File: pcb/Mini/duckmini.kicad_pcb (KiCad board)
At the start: 2 copper layers, 126.9 x 99.3 mm, 42 parts

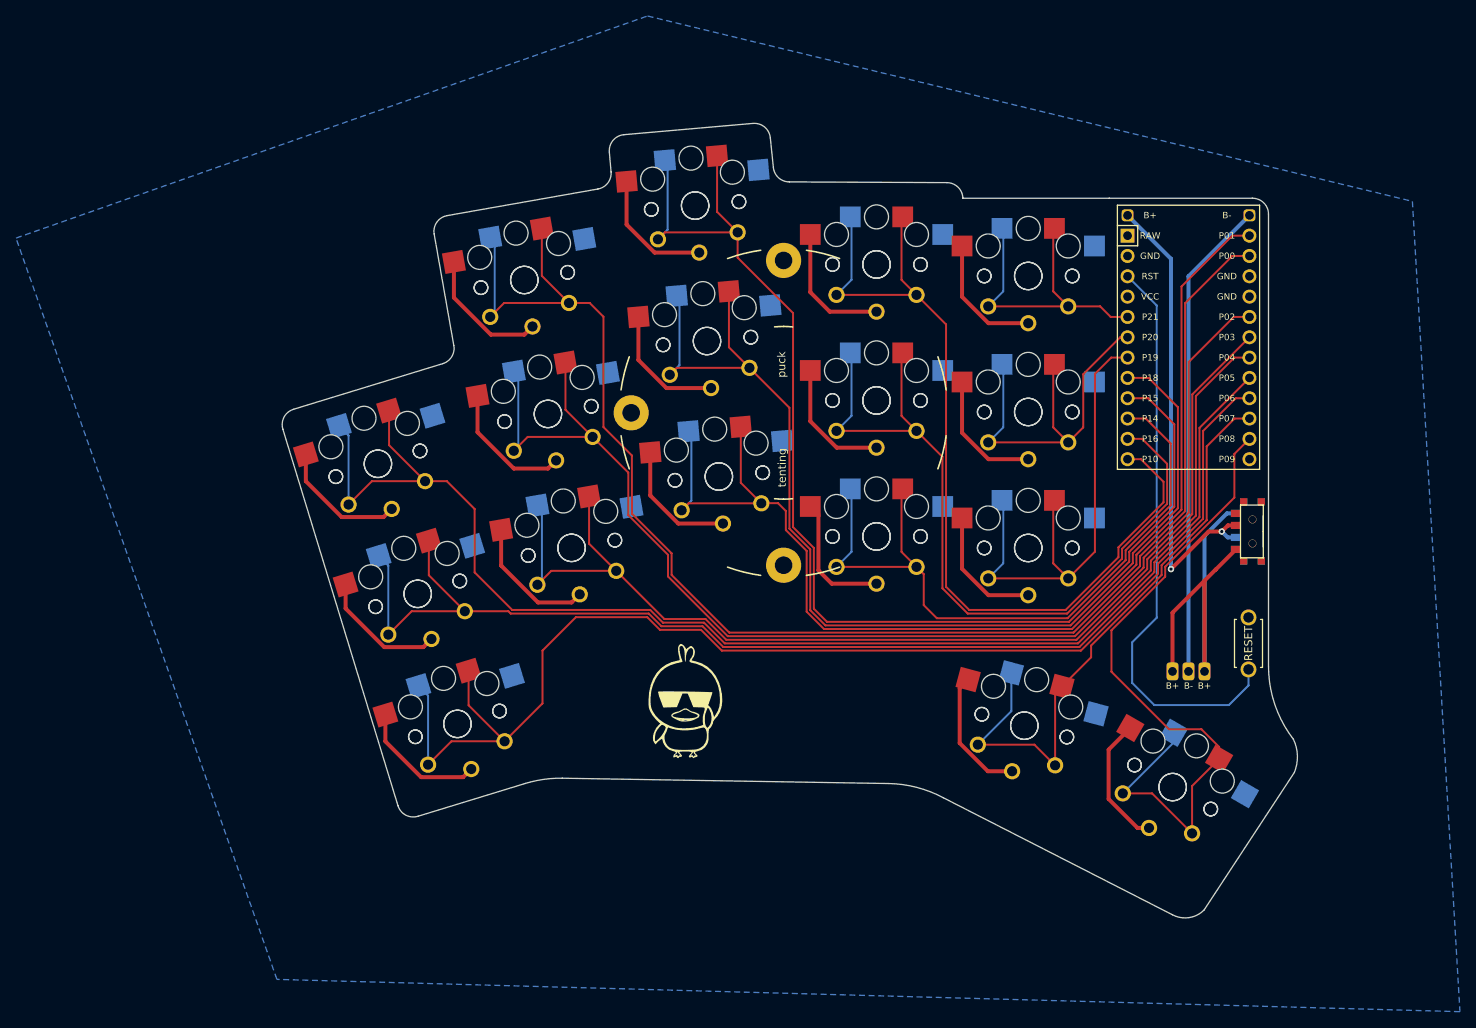
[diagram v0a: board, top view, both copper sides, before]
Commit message: mini
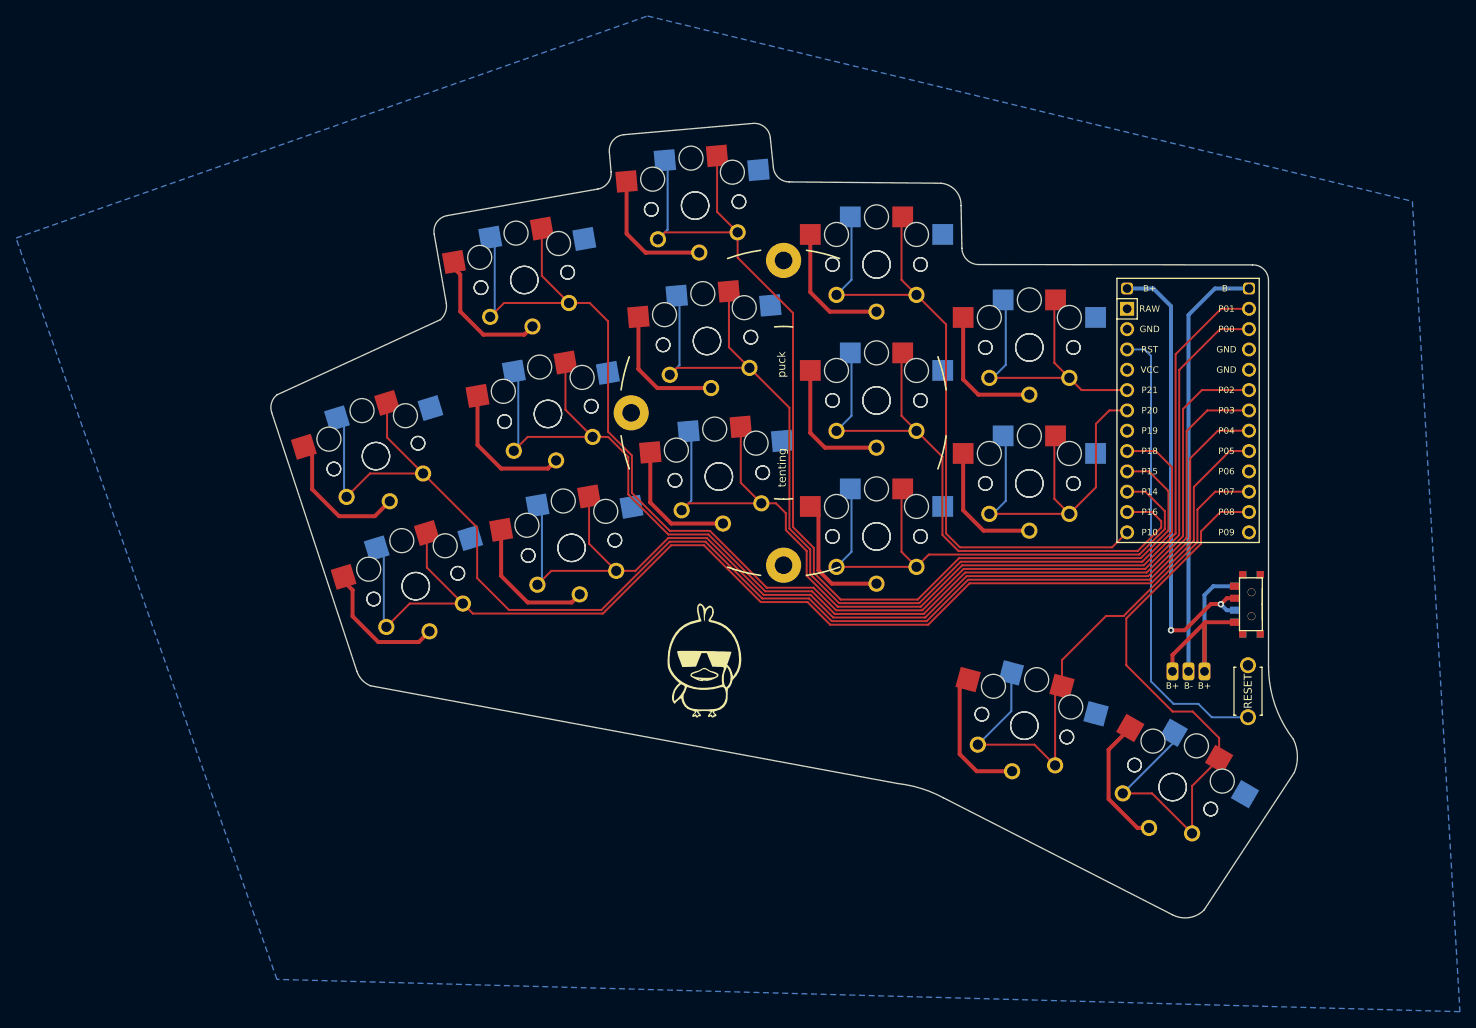
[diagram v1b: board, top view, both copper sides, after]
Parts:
- removed S1, S2, S25, S26: , PG1350
- moved MCU1 9.14 mm to (154.4, -87.2)
- moved T1 9.10 mm to (162.3, -64.2)
- moved T2 9.10 mm to (162.3, -64.2)
- moved S27 8.94 mm to (134.5, -79.3)
- moved S28 8.94 mm to (134.5, -79.3)
- moved S29 8.94 mm to (134.5, -96.3)
- moved S30 8.94 mm to (134.5, -96.3)
- moved B1 5.98 mm to (161.8, -53.3)
- moved G*** 5.68 mm to (94.0, -55.9)
- moved G*** 5.59 mm to (93.8, -55.9)
- moved S5 0.99 mm to (52.8, -82.7)
- moved S6 0.99 mm to (52.8, -82.7)
- moved S3 0.99 mm to (57.8, -66.5)
- moved S4 0.99 mm to (57.8, -66.5)
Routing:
- net P6: track 157.1 -> 0.00 mm
- net P19: track 63.0 -> 0.00 mm
- net P10: track 112.4 -> 87.0 mm
- net Braw: track 51.9 -> 31.4 mm
- net GND: track 274.9 -> 254.5 mm
- net P16: track 99.6 -> 80.8 mm
- net P14: track 89.2 -> 72.5 mm
- net RST: track 72.3 -> 58.0 mm
- net P15: track 152.4 -> 138.4 mm
- net P18: track 138.9 -> 125.3 mm
- net P0: track 183.1 -> 170.0 mm
- net P1: track 142.3 -> 129.4 mm
- net P2: track 157.0 -> 146.5 mm
- net P8: track 86.8 -> 77.3 mm
- net Bminus: track 60.2 -> 53.5 mm
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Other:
- board size 126.9 x 99.3 mm -> 128.3 x 99.3 mm
